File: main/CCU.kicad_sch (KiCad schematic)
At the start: 8 parts, among them U2 ESP32-DevKitC, U27 Oak-D, U4 Waveshare 23721, U5 MPU6050

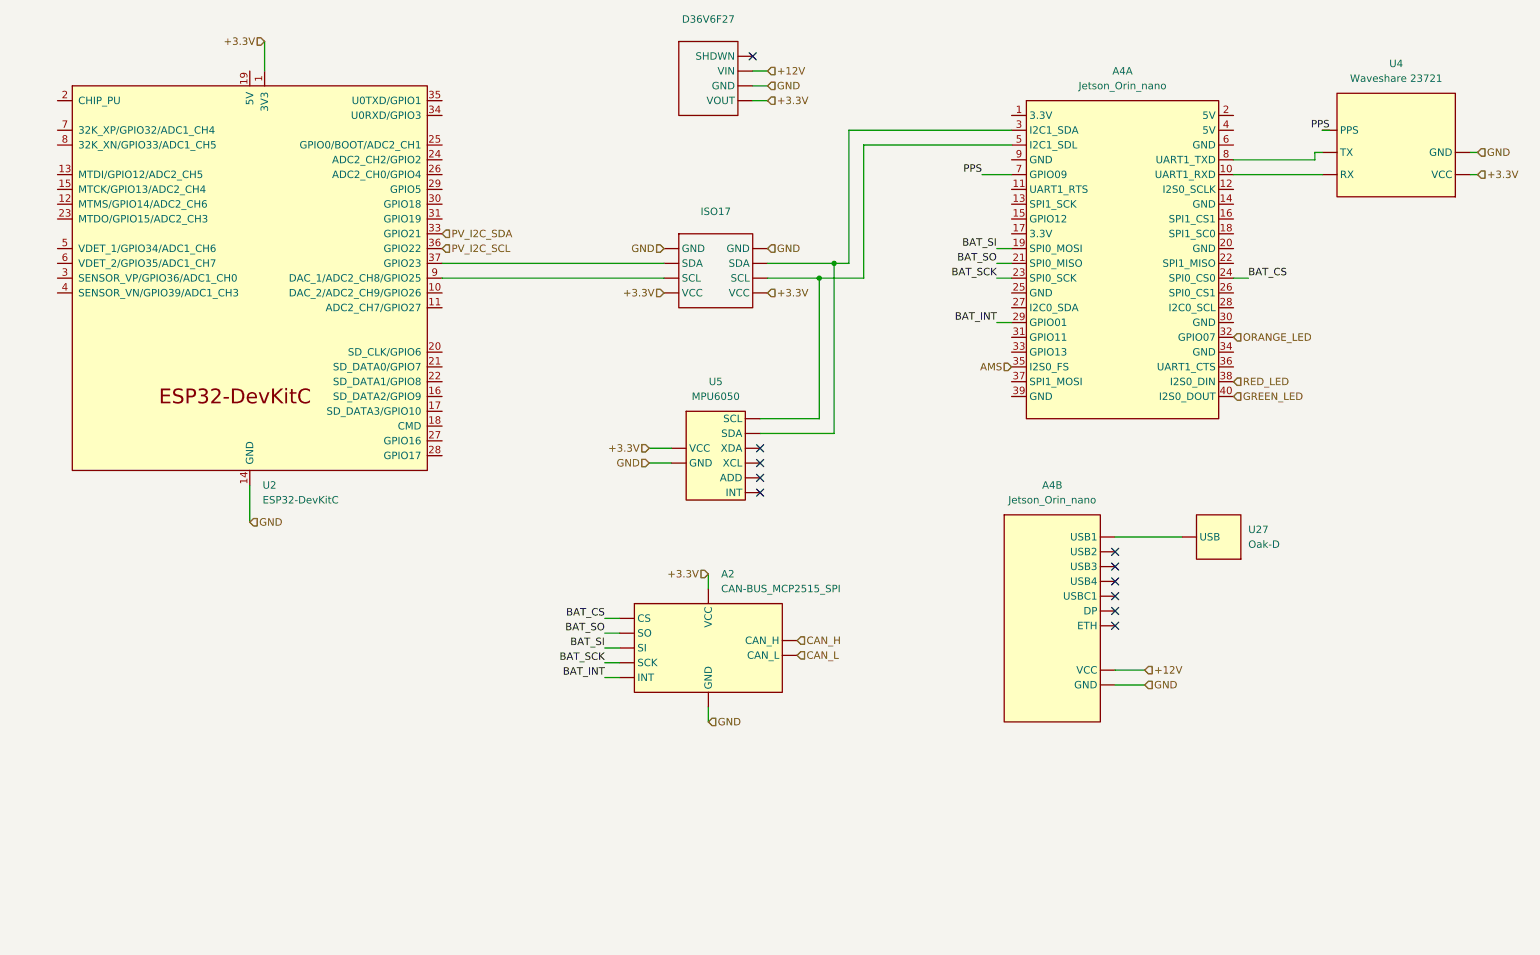
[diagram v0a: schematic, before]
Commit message: added logos, oranised sheets, final version
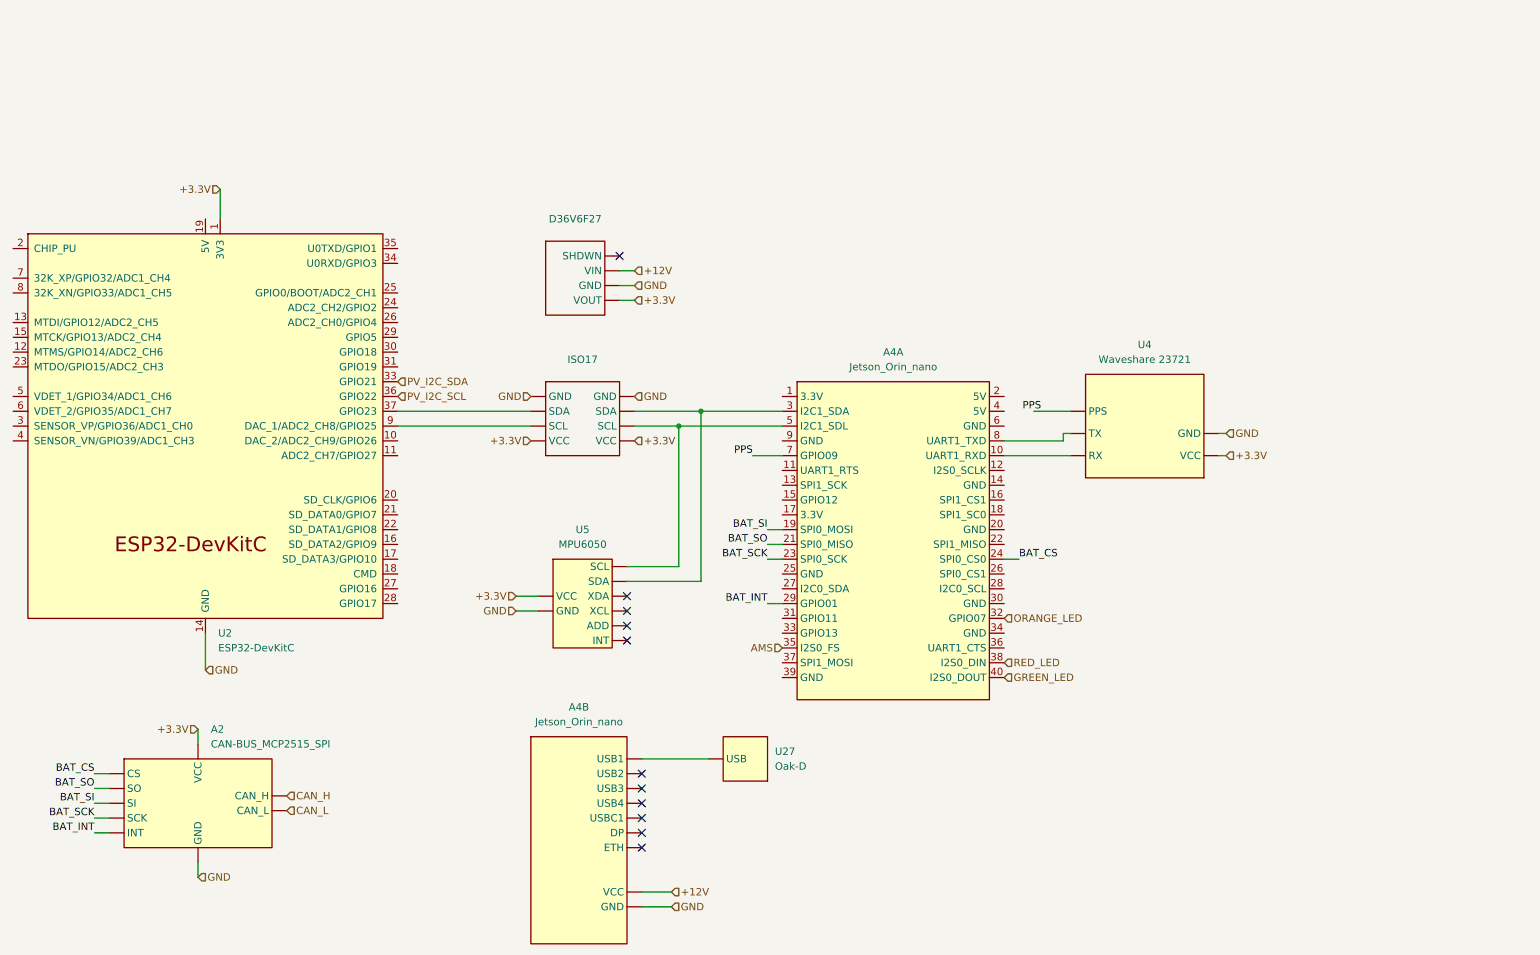
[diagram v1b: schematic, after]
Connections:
- new net: A4.3 (I2C1_SDA), ISO17. (VCC), U5. (XDA)
- new net: A4.5 (I2C1_SDL), ISO17. (VCC), U5. (XDA)
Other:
- company: (none) -> Designers: Krzysztof Grajek, Wojtek Kołodziej
- title: (none) -> Central Control Unit schematic
- moved on the sheet: A2, A4A, A4B, D36V6F27, ISO17, U2, U27, U4, U5
